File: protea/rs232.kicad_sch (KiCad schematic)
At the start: 10 parts, among them J2 D-SUB 9 Male, U6 MAX232CSE+

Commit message: Protea WIP
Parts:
- U6: footprint FRANK:SOIC127P600X175-16N -> FRANK:SOP-16
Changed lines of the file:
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@@
 			)
 		)
-		(property "Footprint" "FRANK:SOIC127P600X175-16N"
+		(property "Footprint" "FRANK:SOP-16"
 			(at 107.95 163.5 0)
 			(effects

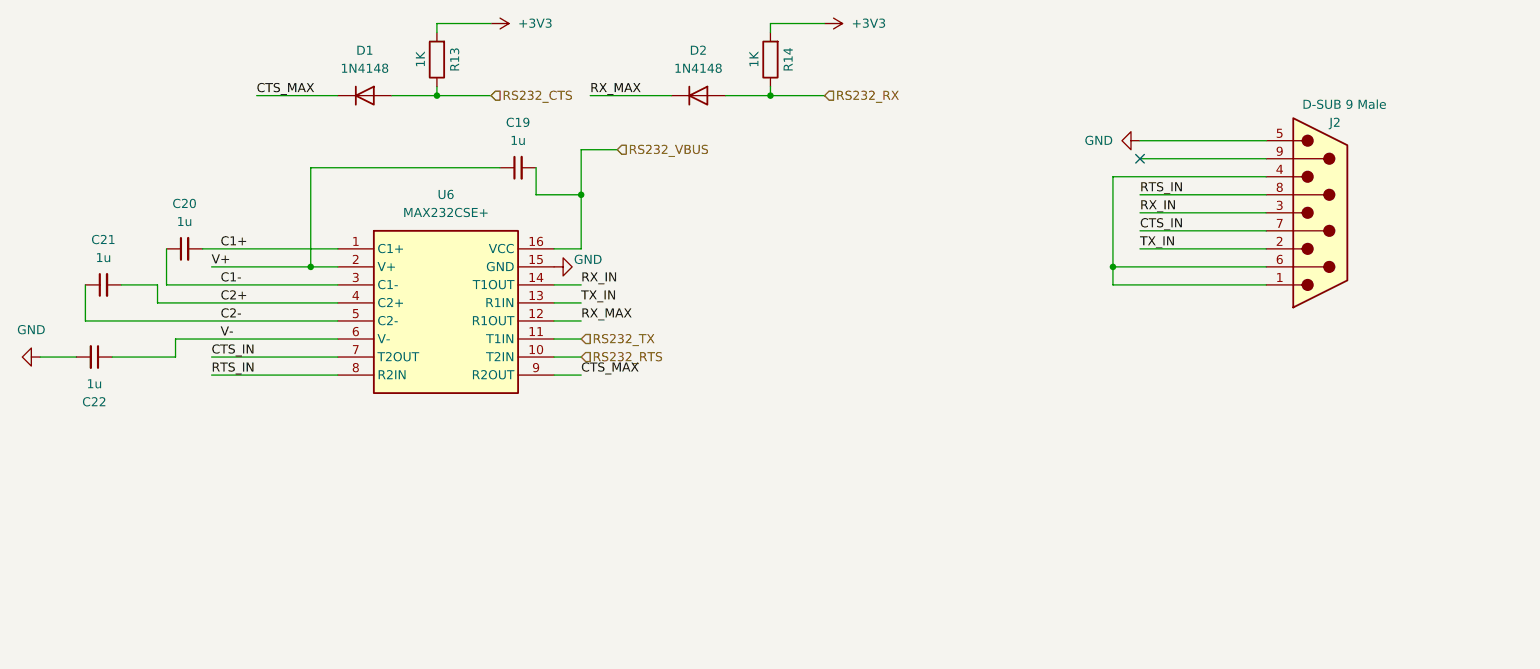
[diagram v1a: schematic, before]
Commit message: Protea HW 2.06
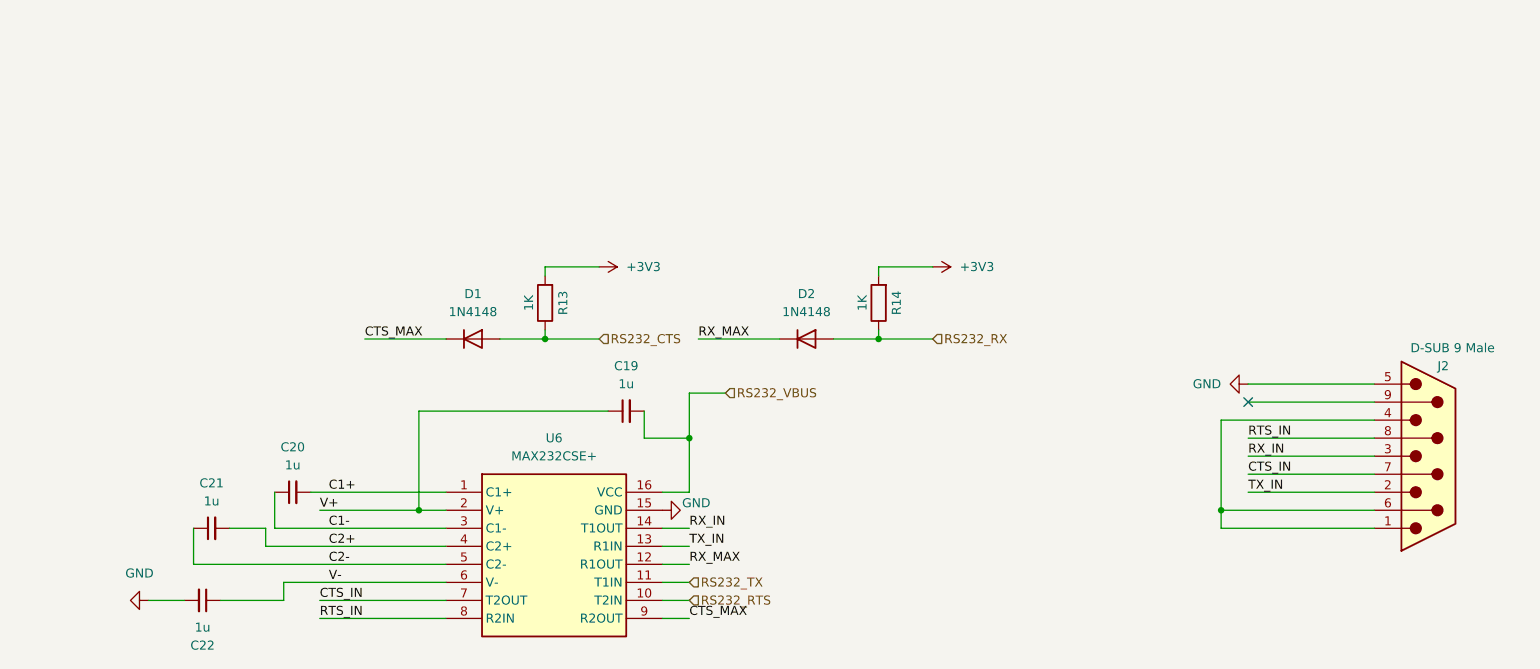
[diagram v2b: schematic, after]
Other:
- moved on the sheet: C19, C20, C21, C22, D1, D2, J2, R13, R14, U6
